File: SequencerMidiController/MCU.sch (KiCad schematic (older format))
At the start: 7 parts, among them U33 STM32G0B1_KxTxN_LQFP32

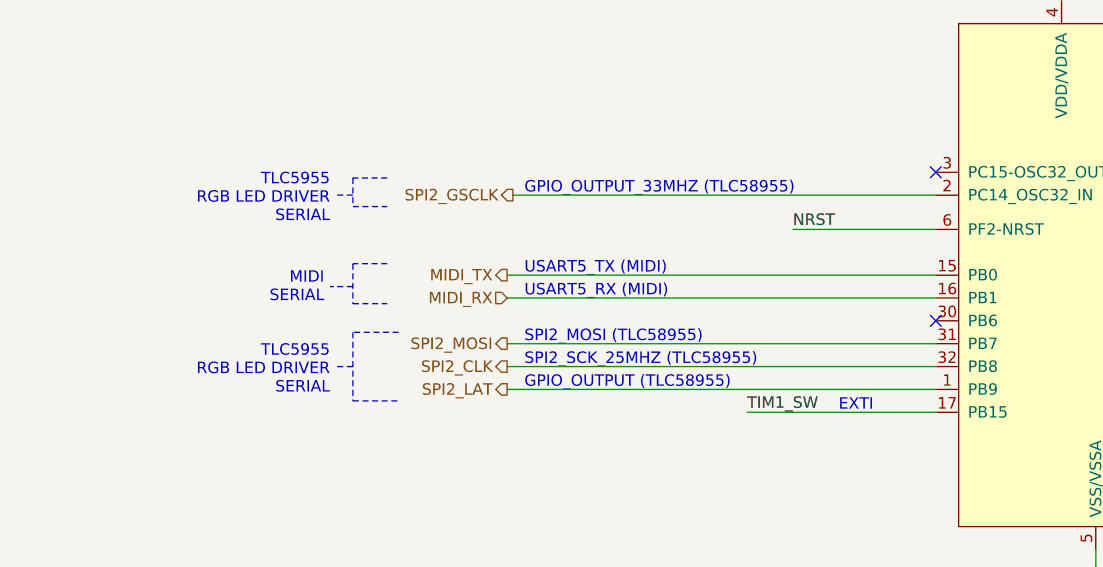
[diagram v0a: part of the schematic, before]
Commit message: updated for kicad 6
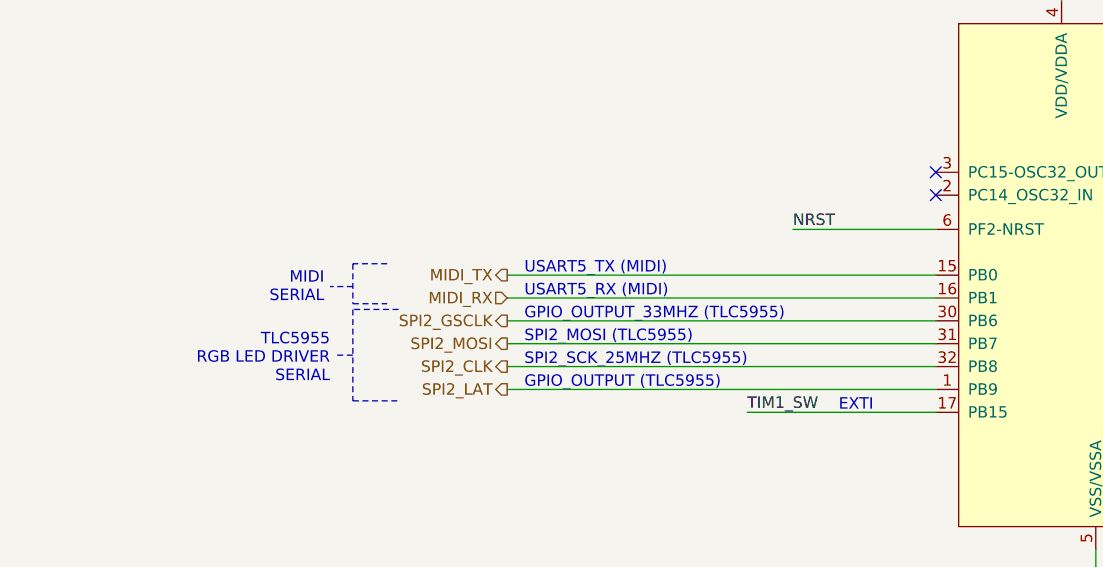
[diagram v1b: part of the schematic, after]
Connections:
- net SPI2_GSCLK: now also U33.30 (PB6); no longer U33.2 (PC14_OSC32_IN)
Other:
- note added: "GPIO_OUTPUT (TLC5955)"
- note added: "GPIO_OUTPUT_33MHZ (TLC5955)"
- note added: "SPI2_MOSI (TLC5955)"
- note added: "SPI2_SCK_25MHZ (TLC5955)"
- note removed: "GPIO_OUTPUT (TLC58955)"
- note removed: "GPIO_OUTPUT_33MHZ (TLC58955)"
- note removed: "SPI2_MOSI (TLC58955)"
- note removed: "SPI2_SCK_25MHZ (TLC58955)"
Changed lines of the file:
@@
 Comment4 ""
 $EndDescr
-$Comp
-L STM32G0B1:STM32G0B1_KxTxN_LQFP32 U33
-U 1 1 60C6B6AE
-P 10475 4425
-F 0 "U33" H 10875 5700 50  0000 C CNN
-F 1 "STM32G0B1_KxTxN_LQFP32" H 11325 5600 50  0000 C CNN
-F 2 "Package_QFP:LQFP-32_7x7mm_P0.8mm" H 10325 4775 50  0001 C CNN
-F 3 "https://www.st.com/resource/en/datasheet/stm32g0b1ke.pdf" H 10325 4775 50  0001 C CNN
-F 4 "~" H 10475 4425 50  0001 C CNN "LcscNo"
-F 5 "~" H 10475 4425 50  0001 C CNN "Type"
-	1    10475 4425
-	1    0    0    -1
-$EndComp
 Wire Wire Line
 	10325 3225 10325 2475
@@
 	9775 4925 7900 4925
 Wire Wire Line
-	9775 4075 7925 4075
+	9775 4625 7900 4625
 Text HLabel 7900 4925 0    50   Output ~ 0
 SPI2_LAT
-Text HLabel 7925 4075 0    50   Output ~ 0
+Text HLabel 7900 4625 0    50   Output ~ 0
 SPI2_GSCLK
 Wire Wire Line
@@
 NoConn ~ 11225 3875
 NoConn ~ 11225 4475
-NoConn ~ 9775 4625
 NoConn ~ 9775 3975
 Text Notes 9225 9625 0    50   ~ 0
@@
 	13450 3600 13525 3600
 Text Notes 7975 4925 0    50   ~ 0
-GPIO_OUTPUT (TLC58955)
+GPIO_OUTPUT (TLC5955)
 Text Notes 7975 4825 0    50   ~ 0
-SPI2_SCK_25MHZ (TLC58955)
+SPI2_SCK_25MHZ (TLC5955)
 Text Notes 7975 4725 0    50   ~ 0
-SPI2_MOSI (TLC58955)
-Text Notes 7975 4075 0    50   ~ 0
-GPIO_OUTPUT_33MHZ (TLC58955)
+SPI2_MOSI (TLC5955)
+Text Notes 7975 4625 0    50   ~ 0
+GPIO_OUTPUT_33MHZ (TLC5955)
 Text Notes 12275 4075 0    50   ~ 0
 I2C3_SDA
@@
 Wire Notes Line
 	13450 4725 13250 4725
-Text Notes 7125 4200 2    50   ~ 0
+Wire Notes Line
+	7425 4575 7225 4575
+Wire Notes Line
+	7225 4575 7225 4975
+Wire Notes Line
+	7225 4975 7425 4975
+Text Notes 7125 4900 2    50   ~ 0
 TLC5955\nRGB LED DRIVER\nSERIAL
 Wire Notes Line
-	7425 4675 7225 4675
-Wire Notes Line
-	7225 4075 7150 4075
-Wire Notes Line
-	7225 4675 7225 4975
-Wire Notes Line
-	7225 4975 7425 4975
-Text Notes 7125 4950 2    50   ~ 0
-TLC5955\nRGB LED DRIVER\nSERIAL
-Wire Notes Line
-	7225 4825 7150 4825
-Wire Notes Line
-	7375 4000 7225 4000
-Wire Notes Line
-	7225 4000 7225 4125
-Wire Notes Line
-	7225 4125 7375 4125
+	7225 4775 7150 4775
 Text Notes 7100 4550 2    50   ~ 0
 MIDI\nSERIAL
@@
 NoConn ~ 11225 5275
 NoConn ~ 11225 5375
+$Comp
+L STM32G0B1:STM32G0B1_KxTxN_LQFP32 U33
+U 1 1 60C6B6AE
+P 10475 4425
+F 0 "U33" H 10875 5700 50  0000 C CNN
+F 1 "STM32G0B1_KxTxN_LQFP32" H 11325 5600 50  0000 C CNN
+F 2 "Package_QFP:LQFP-32_7x7mm_P0.8mm" H 10325 4775 50  0001 C CNN
+F 3 "https://www.st.com/resource/en/datasheet/stm32g0b1ke.pdf" H 10325 4775 50  0001 C CNN
+F 4 "~" H 10475 4425 50  0001 C CNN "LcscNo"
+F 5 "~" H 10475 4425 50  0001 C CNN "Type"
+	1    10475 4425
+	1    0    0    -1
+$EndComp
+NoConn ~ 9775 4075
 $EndSCHEMATC
